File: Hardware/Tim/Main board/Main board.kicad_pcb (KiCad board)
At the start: 4 copper layers, 120.9 x 66.6 mm, 184 parts, among them J1 SOICbite, J10 Conn_01x03_Socket, J11 Conn_01x02_Pin, J12 USB_C_Receptacle_USB2.0, J13 Conn_01x02_Socket, J14 Conn_01x02_Pin, J15 Conn_01x04_Socket, J16 Conn_01x02_Pin, J17 Conn_01x04_Pin, J18 Conn_01x03_Socket, J2 USB_C_Receptacle_USB2.0, J3 Conn_01x04_Socket, J4 Conn_01x04_Socket, J5 Conn_01x04_Socket, J6 Conn_01x02_Socket, J7 Conn_01x02_Socket, J8 U.FL, J9 SOICbite, Q1 IRLML0060TRPBF, Q2 IRLML0060TRPBF, U1 RP2040, U10 MAX-M10S, U11 ADP7105ACPZ-5.0-R7, U12 ADP7105ACPZ-3.3-R7, U13 ADP7105ACPZ-5.0-R7, U14 TPS2121RUXR, U15 TPS2121RUXR, U2 W25Q64JVZP, U3 MS5607-02BA, U4 BMI270, U5 ADP7105ACPZ-3.3-R7, U6 DRF1262TL, U7 RP2040, U8 W25Q64JVZP, Y1 12MHz, Y2 12MHz

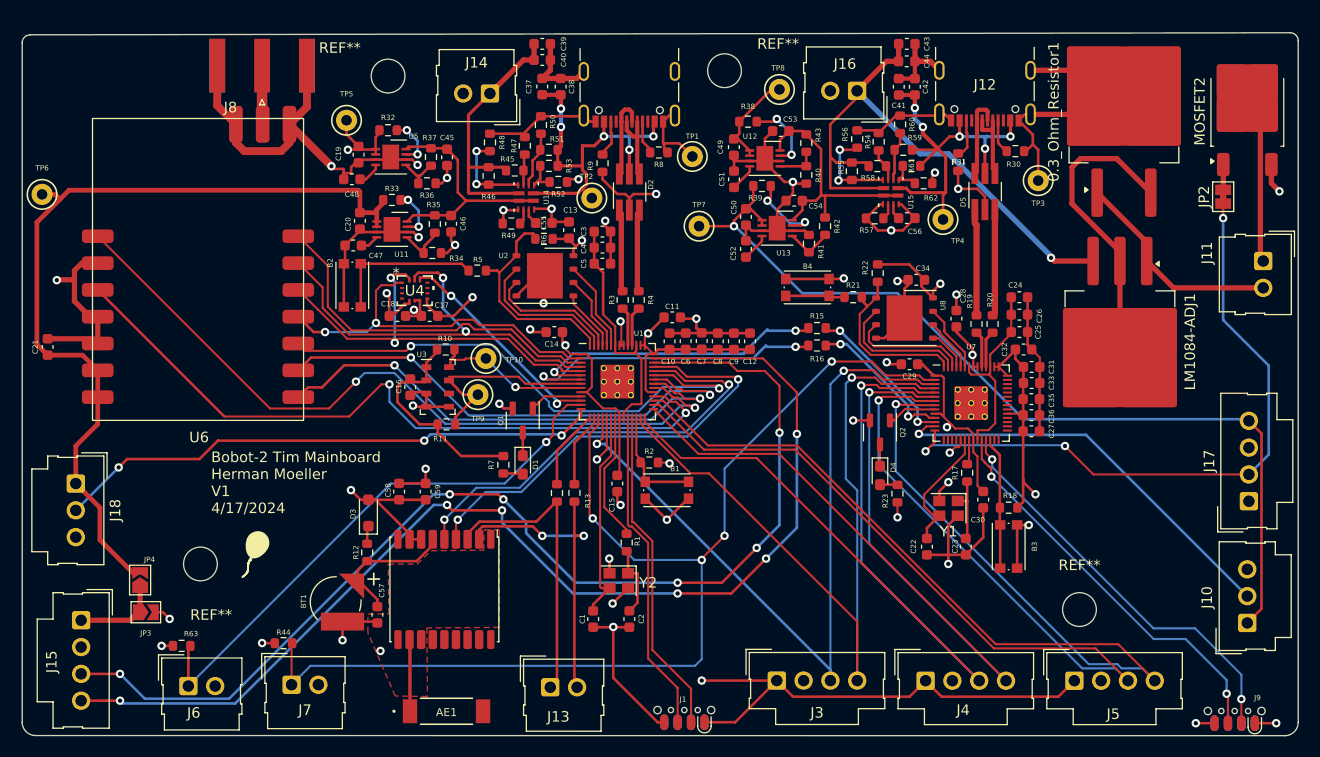
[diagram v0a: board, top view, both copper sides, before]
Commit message: Double checking everything is pushed
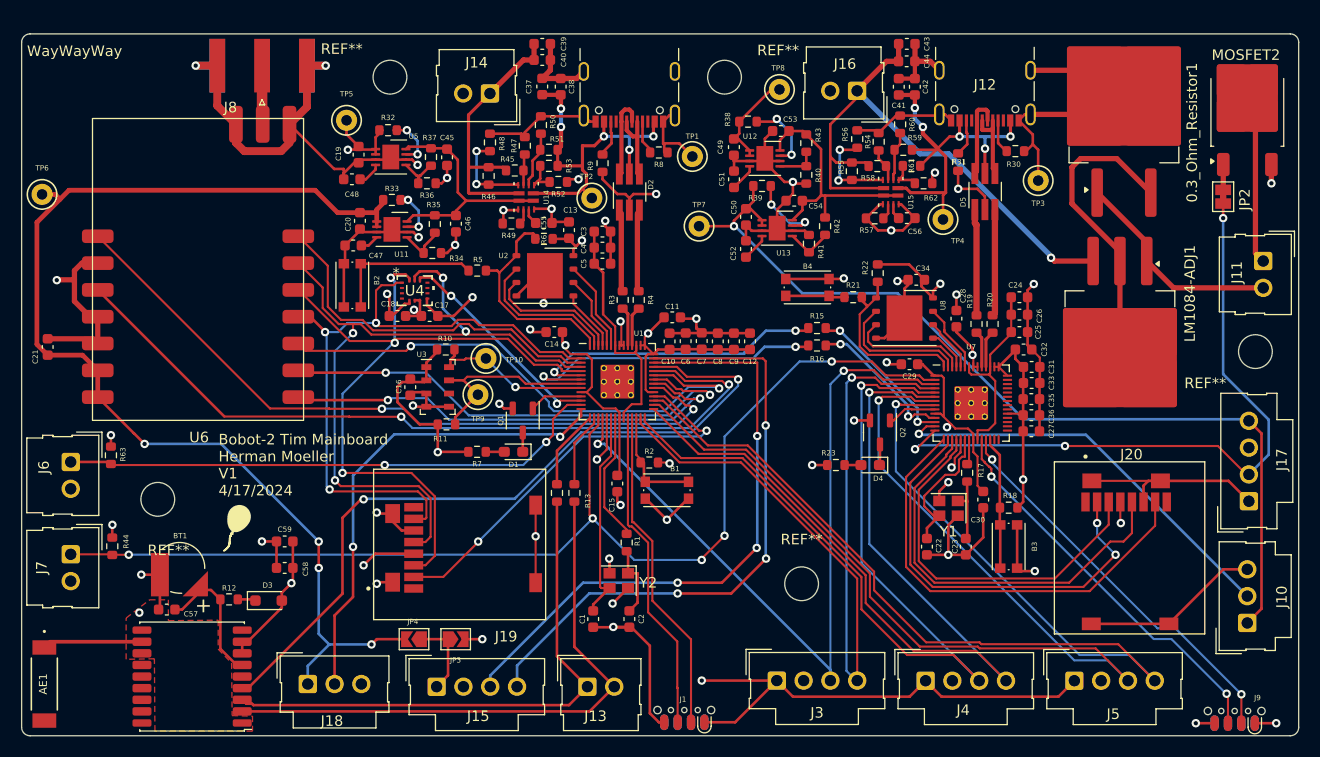
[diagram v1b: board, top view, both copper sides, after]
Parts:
- added J19: Micro_SD_Card, BPPlib:JAE_ST1W008S4ER1500, F.Cu at (99.0, 108.8)
- added J20: Micro_SD_Card, BPPlib:JAE_ST1W008S4ER1500, F.Cu at (154.6, 102.0)
- added REF**: MountingHole_3.2mm_M3, MountingHole:MountingHole_3.2mm_M3, F.Cu at (174.0, 83.0)
- moved AE1 38.2 mm to (59.2, 114.5), turned to -90 degrees
- moved J15 34.3 mm to (96.4, 114.8), turned to 0 degrees
- moved JP3 29.5 mm to (98.2, 110.2)
- moved J18 29.1 mm to (84.2, 114.5), turned to 0 degrees
- moved JP4 26.5 mm to (94.3, 110.2), turned to 180 degrees
- moved REF** 26.4 mm to (131.0, 105.0)
- moved U10 25.3 mm to (73.2, 113.8), turned to 180 degrees
- moved J7 24.3 mm to (61.8, 102.2), turned to -90 degrees
- moved J6 24.0 mm to (61.8, 93.5), turned to -90 degrees
- moved C57 20.0 mm to (70.8, 107.4), turned to 180 degrees
- moved R63 19.3 mm to (65.6, 92.8), turned to -90 degrees
- moved R44 18.6 mm to (65.7, 101.4), turned to -90 degrees
- moved BT1 15.2 mm to (72.1, 103.5), turned to -90 degrees
- moved C59 14.2 mm to (82.0, 101.0), turned to 180 degrees
- moved R12 13.8 mm to (76.8, 106.5), turned to 180 degrees
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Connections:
- U1 pad 32: /TXEN -> /SPI0_CS_SD
- U1 pad 38: /EXTINT -> /TXEN
- U7 pad 15: unconnected-(U7-GPIO12-Pad15) -> /SPI0_POCI_R
- U7 pad 16: unconnected-(U7-GPIO13-Pad16) -> /SPI0_CS_SD_R
- U7 pad 17: unconnected-(U7-GPIO14-Pad17) -> /SPI0_SCK_R
- U7 pad 18: unconnected-(U7-GPIO15-Pad18) -> /SPI0_PICO_R
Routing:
- net /DIR: track 110.2 -> 59.2 mm, vias 6 -> 3
- net /STEP: track 107.7 -> 58.7 mm, vias 6 -> 3
- net GND: track 335.8 -> 384.0 mm, vias 41 -> 46
- net /SPI0_POCI_R: track 0.00 -> 42.9 mm
- net /EXTINT: track 42.0 -> 0.00 mm, vias 2 -> 0
- net /SPI0_CS_SD_R: track 0.00 -> 40.7 mm, vias 0 -> 2
- net /SPI0_CS_SD: track 0.00 -> 39.9 mm, vias 0 -> 2
- net /SPI0_SCK_R: track 0.00 -> 39.5 mm
- net /SPI0_PICO_R: track 0.00 -> 36.0 mm
- net /SPI0_PICO: track 39.1 -> 71.4 mm, vias 2 -> 3
- net /SPI0_SCK: track 41.8 -> 72.6 mm, vias 2 -> 4
- net /TIMEPULSE: track 42.9 -> 71.6 mm
- net +5V: track 81.5 -> 108.5 mm, vias 0 -> 4
- net /SPI0_POCI: track 35.5 -> 62.0 mm, vias 2 -> 3
- net Net-(J13-Pin_2): track 29.9 -> 55.3 mm, vias 2 -> 0
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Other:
- board size 120.9 x 66.6 mm -> 121 x 66.5 mm
- board text added: "WayWayWay"
